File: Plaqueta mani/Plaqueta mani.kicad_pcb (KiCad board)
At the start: 2 copper layers, 99.9 x 92.7 mm, 33 parts, among them J1 Arduino_Nano_Header, J1 HEADER_8, J2 Alimentacion +5v, J3 HEADER_8, J5 Motor A, J6 Motor B, P1 Modulo Qre113, P1 Modulo_QRE113, SW2 SW_SPDT, U1 QRE1113, U2 QRE1113, U3 QRE1113, U4 QRE1113, U5 QRE1113, U6 QRE1113

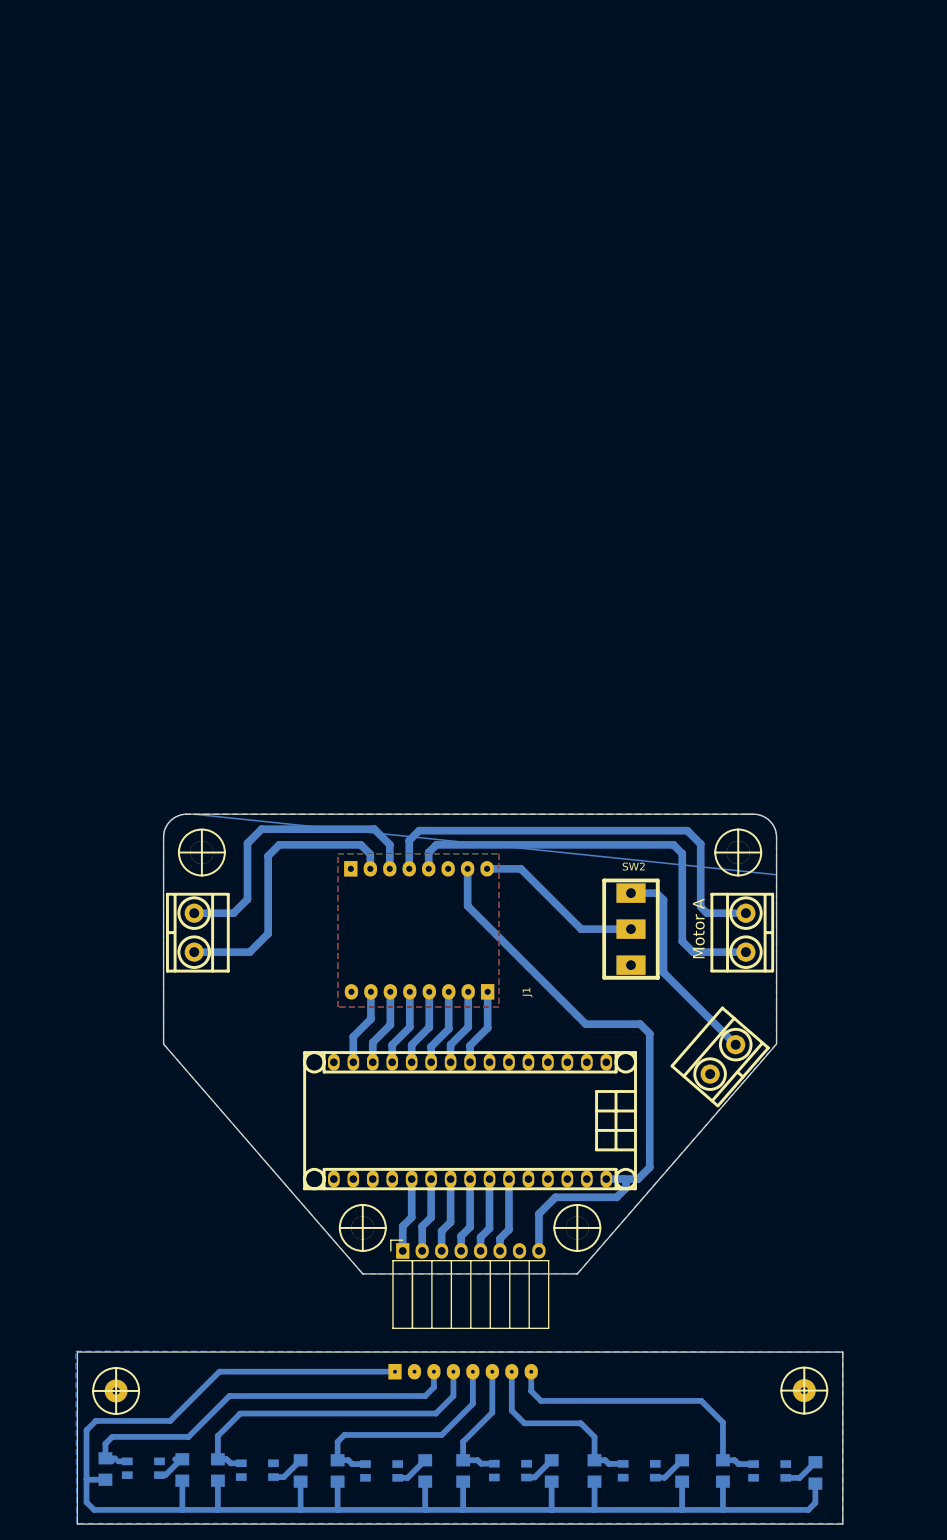
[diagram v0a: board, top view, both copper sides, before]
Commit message: Add files via upload
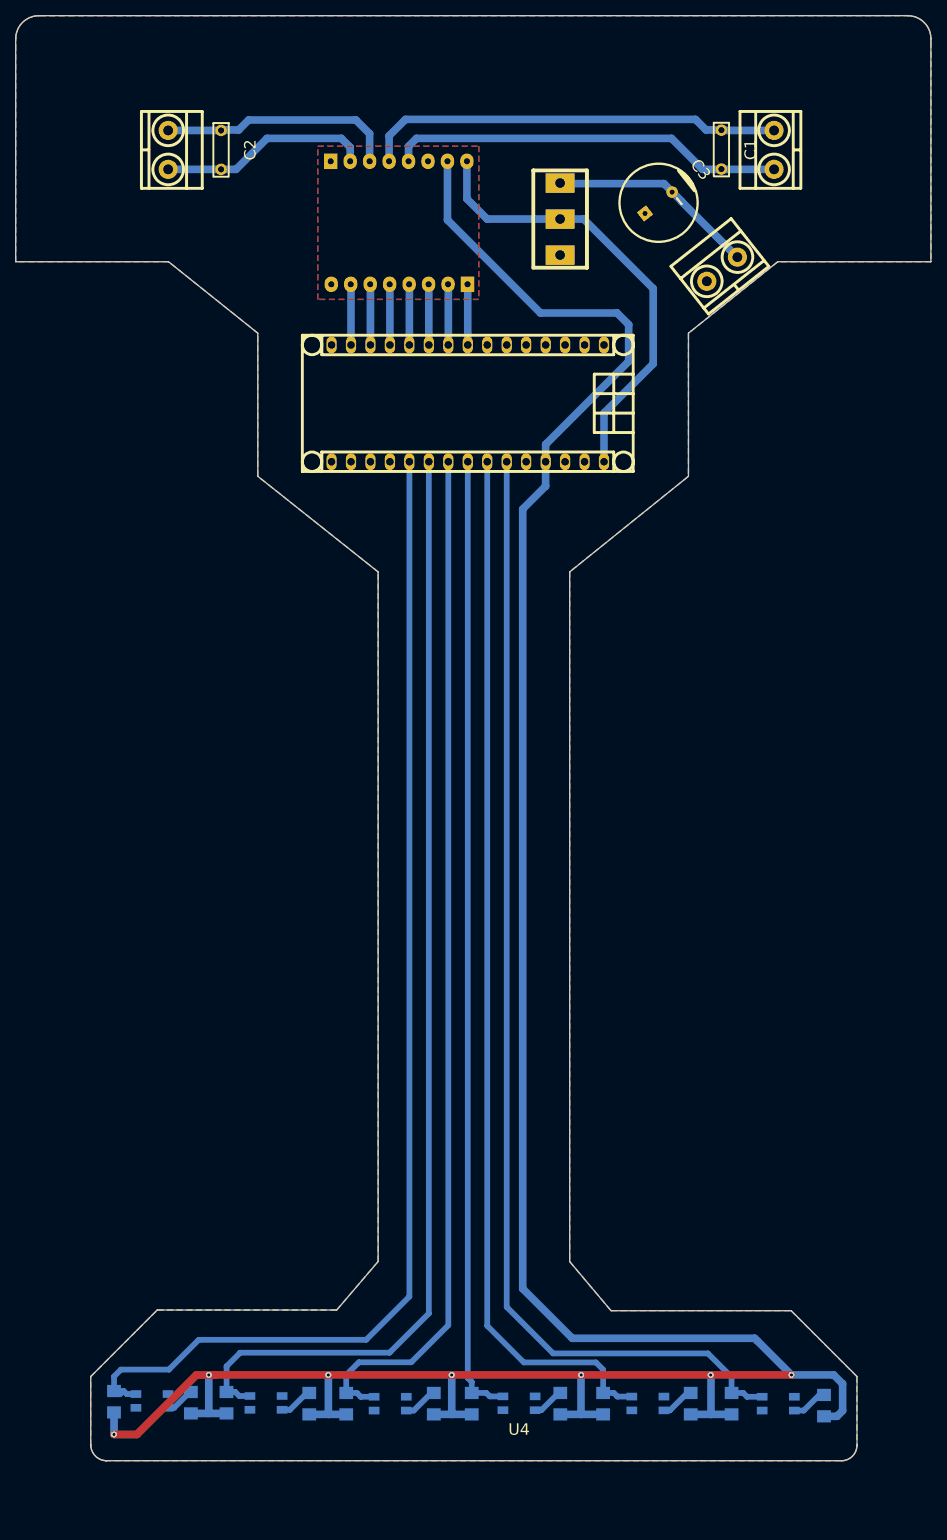
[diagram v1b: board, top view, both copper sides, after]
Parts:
- removed H1 (x2), H2 (x2), H3, H4: Mounting_Hole, EESTN5:hole_3mm
- removed P1: Modulo_QRE113, EESTN5:Socket_Strip_Angled_1x08
- removed P1: Modulo Qre113, EESTN5:Pin_Header_Straight_1x08
- added C1: 0.1uf, EESTN5:CAP_0.2, F.Cu at (159.8, 31.3)
- added C2: 0.1uf, EESTN5:CAP_0.2, F.Cu at (94.5, 31.3)
- added C3: C, EESTN5:CAP_ELEC_10X8mm, F.Cu at (151.6, 38.2)
- J2: value Alimentacion +5v -> Alimentacion +7.5v
- moved J2 103.1 mm to (159.9, 46.9), turned to 38.3 degrees
- moved J5 102.2 mm to (166.7, 31.3)
- moved J6 102.2 mm to (87.6, 31.3)
- moved J1 93.6 mm to (126.7, 64.4)
- moved SW2 93.1 mm to (138.8, 40.3)
- moved J3 92.4 mm to (117.7, 32.8)
- moved J1 92.4 mm to (117.8, 48.8)
- moved R10 8.85 mm to (144.4, 194.9)
- moved R2 8.85 mm to (106.0, 194.9)
- moved R5 8.85 mm to (122.3, 194.9)
- moved R7 8.85 mm to (138.8, 194.9)
- moved R9 8.85 mm to (155.8, 194.9)
- moved U1 8.85 mm to (100.4, 194.8)
- moved U3 8.85 mm to (116.6, 194.9)
- moved R4 8.85 mm to (80.5, 194.7)
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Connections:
- J1 pad 20: /QR_6 -> /QR_1
- J1 pad 21: /QR_5 -> /QR_2
- J1 pad 22: /QR_4 -> /QR_3
- J1 pad 23: /QR_3 -> /QR_4
- J1 pad 24: /QR_2 -> /QR_5
- J1 pad 25: /QR_1 -> /QR_6
- J1 pad 27: unconnected-(J1-5V-Pad27) -> +5V
- J1 pad 30: +5V -> +7.5V
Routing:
- net /QR_5: track 34.1 -> 137.3 mm
- net /QR_6: track 48.2 -> 149.7 mm
- net +5V: track 269.1 -> 368.7 mm, vias 0 -> 7
- net /QR_4: track 27.3 -> 126.0 mm
- net /QR_3: track 40.0 -> 134.9 mm
- net /QR_2: track 52.3 -> 147.0 mm
- net /QR_1: track 62.7 -> 157.3 mm
- net +7.5V: track 22.0 -> 59.3 mm
- net /BO1: track 37.1 -> 27.7 mm
- net /BO2: track 38.4 -> 31.2 mm
- net /AO1: track 56.5 -> 51.8 mm
- net Net-(SW2-A): track 27.4 -> 31.6 mm
- net /BI2: track 10.7 -> 7.93 mm
- net /AO2: track 57.4 -> 55.1 mm
- net /STBY: track 10.2 -> 7.94 mm
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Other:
- board size 99.9 x 92.7 mm -> 119.5 x 188.6 mm
